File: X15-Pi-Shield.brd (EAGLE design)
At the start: 160 x 100 mm, 70 parts, among them J1 T2I, J2 T2I, J3 DF13-4P-1.25DSA, J4 T2I, J5 DF13-4P-1.25DSA, J6 DF13-4P-1.25DSA, Q1 220mA/50V/3.5Ω, Q2 2.5A/30V/105mΩ, Q3 220mA/50V/3.5Ω, Q4 220mA/50V/3.5Ω, Q5 220mA/50V/3.5Ω, U1 ULN2003AD, U2 MAX1136EUA-T, Y2 ECS-80-S-4X

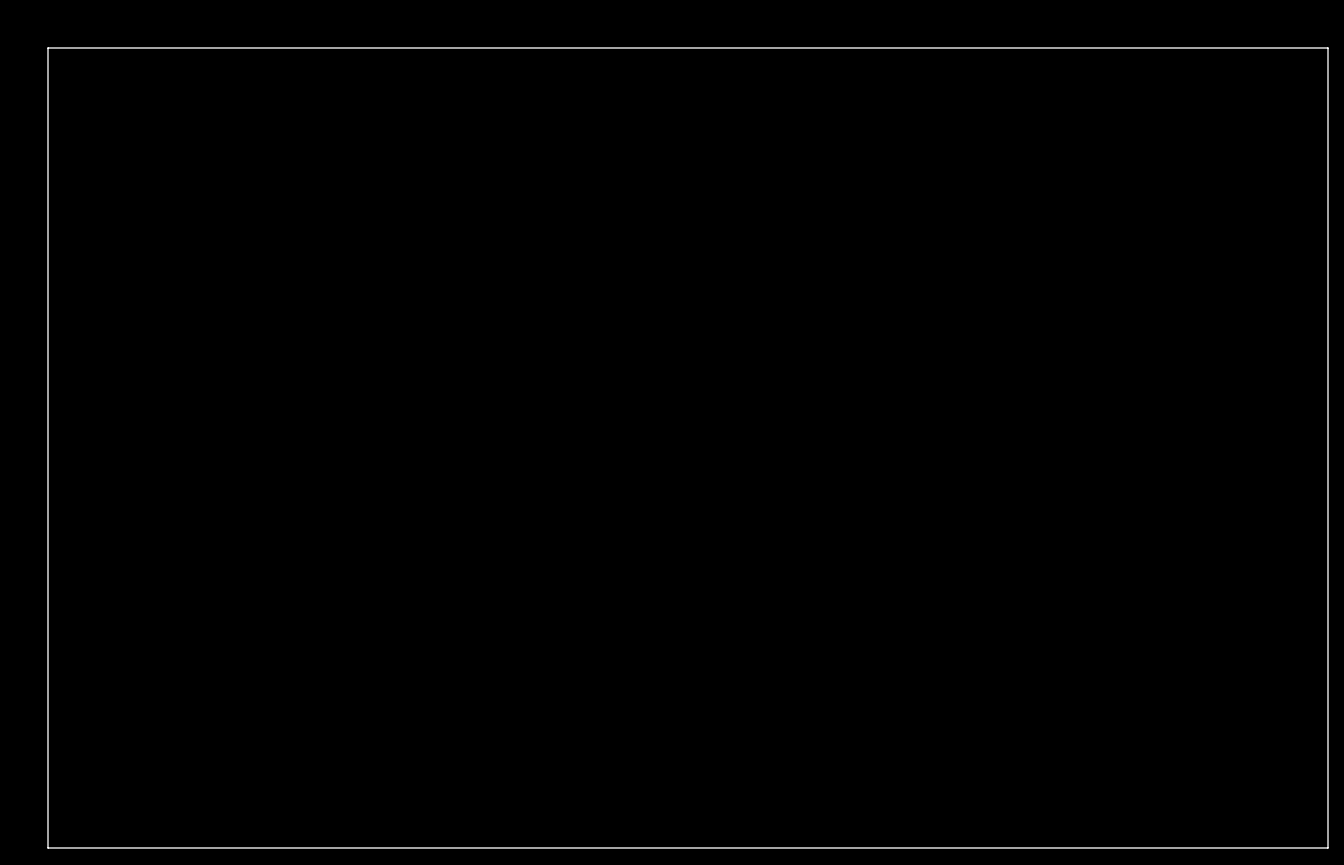
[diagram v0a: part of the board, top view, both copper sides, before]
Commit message: Board Dimensions AGAIN
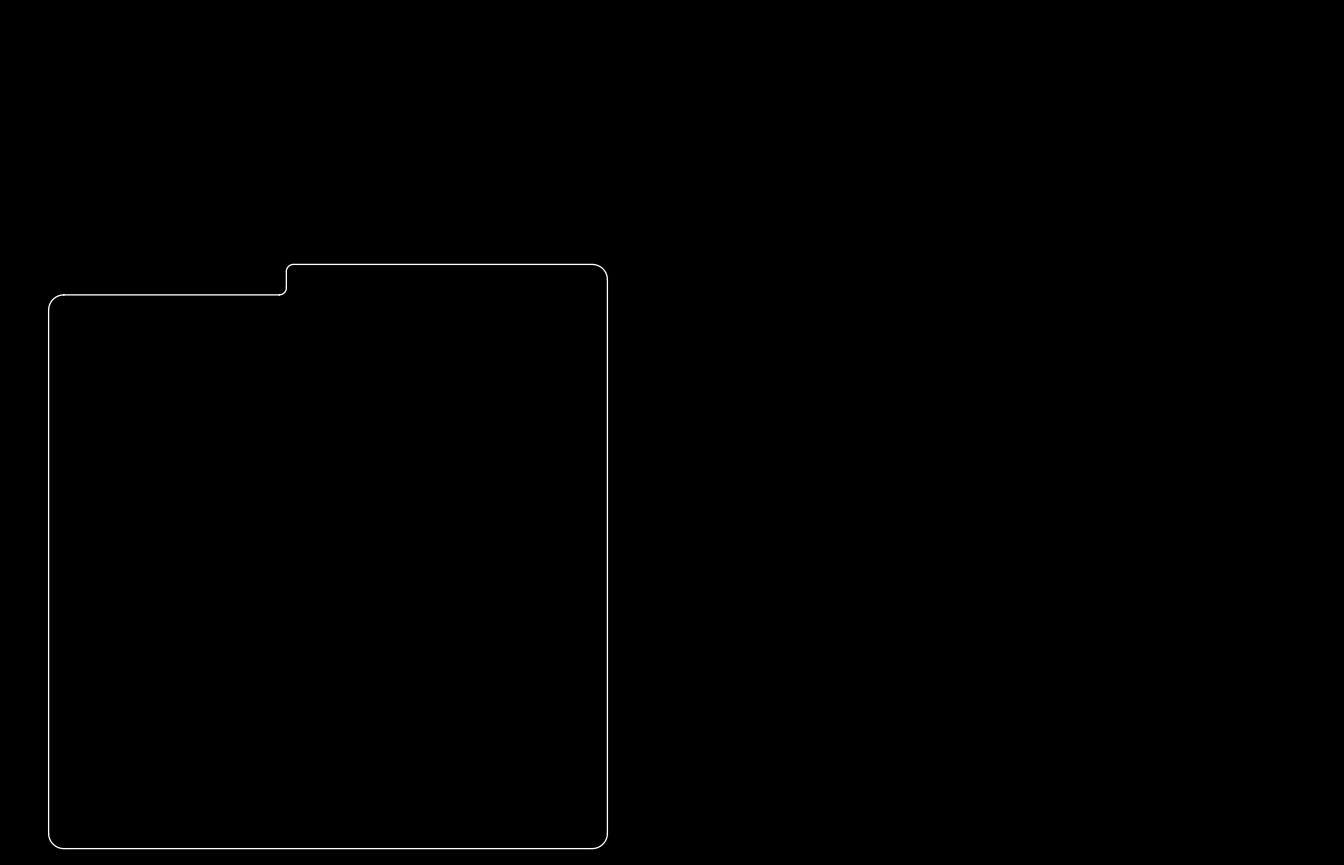
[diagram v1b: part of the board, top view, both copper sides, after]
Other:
- board size 160 x 100 mm -> 69.8 x 73 mm
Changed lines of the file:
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@@
 <setting verticaltext="up"/>
 </settings>
-<grid distance="50" unitdist="mil" unit="mil" style="lines" multiple="1" display="no" altdistance="5" altunitdist="mil" altunit="mil"/>
+<grid distance="1" unitdist="mil" unit="mil" style="lines" multiple="1" display="no" altdistance="5" altunitdist="mil" altunit="mil"/>
 <layers>
 <layer number="1" name="Top" color="4" fill="1" visible="yes" active="yes"/>
@@
 <layer number="154" name="FabDoc2" color="7" fill="1" visible="yes" active="yes"/>
 <layer number="155" name="FabDoc3" color="7" fill="1" visible="yes" active="yes"/>
+<layer number="166" name="AntennaArea" color="7" fill="1" visible="yes" active="yes"/>
+<layer number="168" name="4mmHeightArea" color="7" fill="1" visible="yes" active="yes"/>
 <layer number="191" name="mNets" color="7" fill="1" visible="yes" active="yes"/>
 <layer number="192" name="mBusses" color="7" fill="1" visible="yes" active="yes"/>
@@
 <board>
 <plain>
-<wire x1="0" y1="0" x2="160" y2="0" width="0" layer="20"/>
-<wire x1="160" y1="0" x2="160" y2="100" width="0" layer="20"/>
-<wire x1="160" y1="100" x2="0" y2="100" width="0" layer="20"/>
-<wire x1="0" y1="100" x2="0" y2="0" width="0" layer="20"/>
+<wire x1="1.9812" y1="69.1388" x2="28.9052" y2="69.1388" width="0.1524" layer="20"/>
+<wire x1="28.9052" y1="69.1388" x2="29.7942" y2="70.0278" width="0.1524" layer="20" curve="90"/>
+<wire x1="29.7942" y1="70.0278" x2="29.7942" y2="72.0598" width="0.1524" layer="20"/>
+<wire x1="29.7942" y1="72.0598" x2="30.6832" y2="72.9488" width="0.1524" layer="20" curve="-90"/>
+<wire x1="30.6832" y1="72.9488" x2="68.0212" y2="72.9488" width="0.1524" layer="20"/>
+<wire x1="68.0212" y1="72.9488" x2="69.9262" y2="71.0438" width="0.1524" layer="20" curve="-90"/>
+<wire x1="69.9262" y1="71.0438" x2="69.9262" y2="1.8288" width="0.1524" layer="20"/>
+<wire x1="69.9262" y1="1.8288" x2="68.0212" y2="-0.0762" width="0.1524" layer="20" curve="-90"/>
+<wire x1="68.0212" y1="-0.0762" x2="1.9812" y2="-0.0762" width="0.1524" layer="20"/>
+<wire x1="1.9812" y1="-0.0762" x2="0.0762" y2="1.8288" width="0.1524" layer="20" curve="-90"/>
+<wire x1="0.0762" y1="1.8288" x2="0.0762" y2="67.2338" width="0.1524" layer="20"/>
+<wire x1="0.0762" y1="67.2338" x2="1.9812" y2="69.1388" width="0.1524" layer="20" curve="-90"/>
 </plain>
 <attributes>
